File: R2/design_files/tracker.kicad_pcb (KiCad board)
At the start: 4 copper layers, 49.4 x 53.4 mm, 97 parts, among them J1 Conn_01x01, J2 Conn_01x01, J3 Conn_01x05, J4 Conn_Coaxial, J5 SIM_Card, J6 Conn_01x02, M1 BG96, Q1 DMP2008UFG, U1 STM32U545CEUx, U10 PUMH10,115, U11 BQ25622E, U12 MC3479, U13 PUMH10,115, U2 GD25QxxxEY, U3 PUMH10,115, U4 NXB0108PW, U5 AP22800HB-7, U6 DF6A6.8FUT, U7 PUMH10,115, U8 LMR51430, U9 AP61100Z6, Y1 32.768KHz, Y2 8MHz

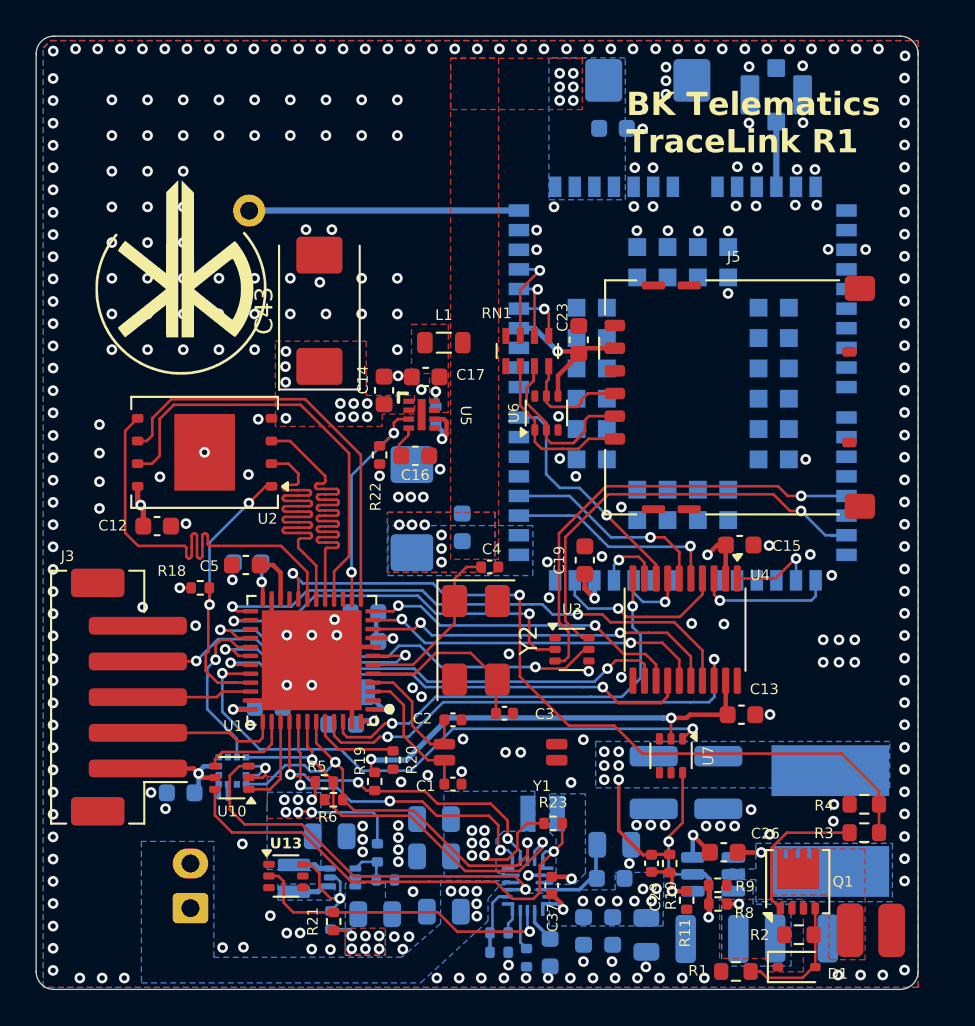
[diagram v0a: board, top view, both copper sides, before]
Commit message: Refactor code structure for improved readability and maintainability
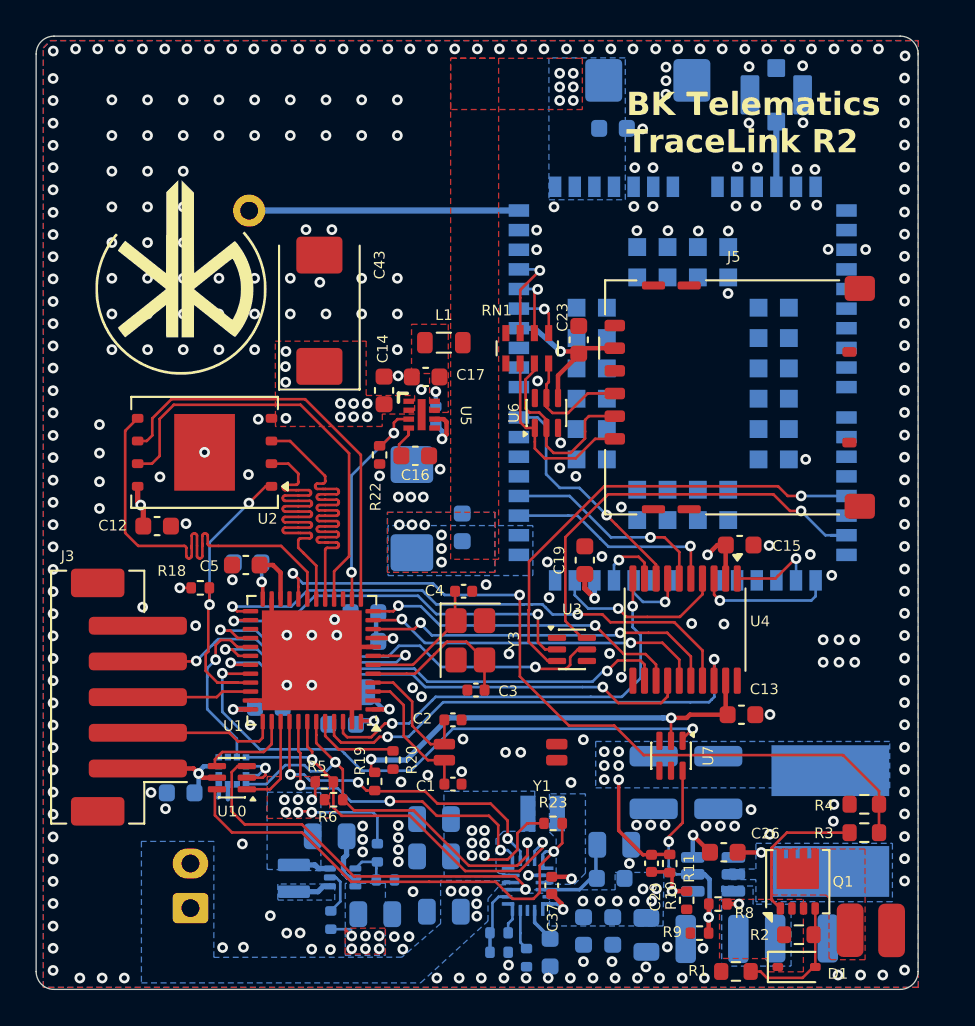
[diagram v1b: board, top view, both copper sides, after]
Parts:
- removed R21: 10K, Resistor_SMD:R_0402_1005Metric
- removed U13: PUMH10,115, Package_TO_SOT_SMD:SOT-363_SC-70-6
- removed Y2: 8MHz, Crystal:Crystal_SMD_0603-4Pin_6.0x3.5mm
- added Y3: 8MHz, Crystal:Crystal_SMD_SeikoEpson_FA238-4Pin_3.2x2.5mm, F.Cu at (146.9, 77.0)
- U11: value BQ25622E -> Untitled_1
- moved R9 2.87 mm to (159.7, 93.4), turned to 0 degrees
- moved C3 2.06 mm to (147.2, 79.8), turned to 0 degrees
- moved C4 2.00 mm to (146.5, 74.2)
- moved RN1 0.16 mm to (150.1, 60.6)
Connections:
- U11 pad 3: /battery charger/CHARGER_PG -> unconnected-(U11-~{PG}-Pad3)
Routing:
- net /battery charger/CHARGER_PG: track 17.8 -> 0.00 mm, vias 1 -> 0
- net Net-(U9-EN): track 5.85 -> 2.54 mm, vias 1 -> 0
- net GND: track 19.4 -> 22.3 mm, vias 317 -> 321
- net /mcu/OSC_OUT: track 9.90 -> 7.20 mm
- net Net-(J5-I/O): track 9.32 -> 12.0 mm
- net Net-(J5-CLK): track 8.95 -> 10.8 mm
- net /gsm/PWRKEY: track 25.4 -> 26.8 mm
- net /gsm/GSM_PWRKEY: track 24.3 -> 25.5 mm
- net /mcu/OSC_IN: track 9.98 -> 9.10 mm
- net +VSYS: track 7.10 -> 6.39 mm
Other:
- board text added: "BK Telematics TraceLink R2"
- board text removed: "BK Telematics TraceLink R1"
